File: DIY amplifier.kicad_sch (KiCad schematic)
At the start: 87 parts, among them J1 AudioPlug3, J2 Output, J3 Input, Q1 IRF540N, Q2 IRF540N, Q3 IRF540N, Q4 IRF540N, Q5 DMN2310U, Q6 BC858, Q7 BC858, Q8 BC848, Q9 BC858, SW1 Reset, U1 74LVC1G14, U10 INA181, U11 74LVC2G17, U2 OPA310SxDBV, U3 HIP4081A, U4 74LVC1G17, U5 L7805, U6 L7812, U7 TLV3501AIDBV, U8 MCP6561U

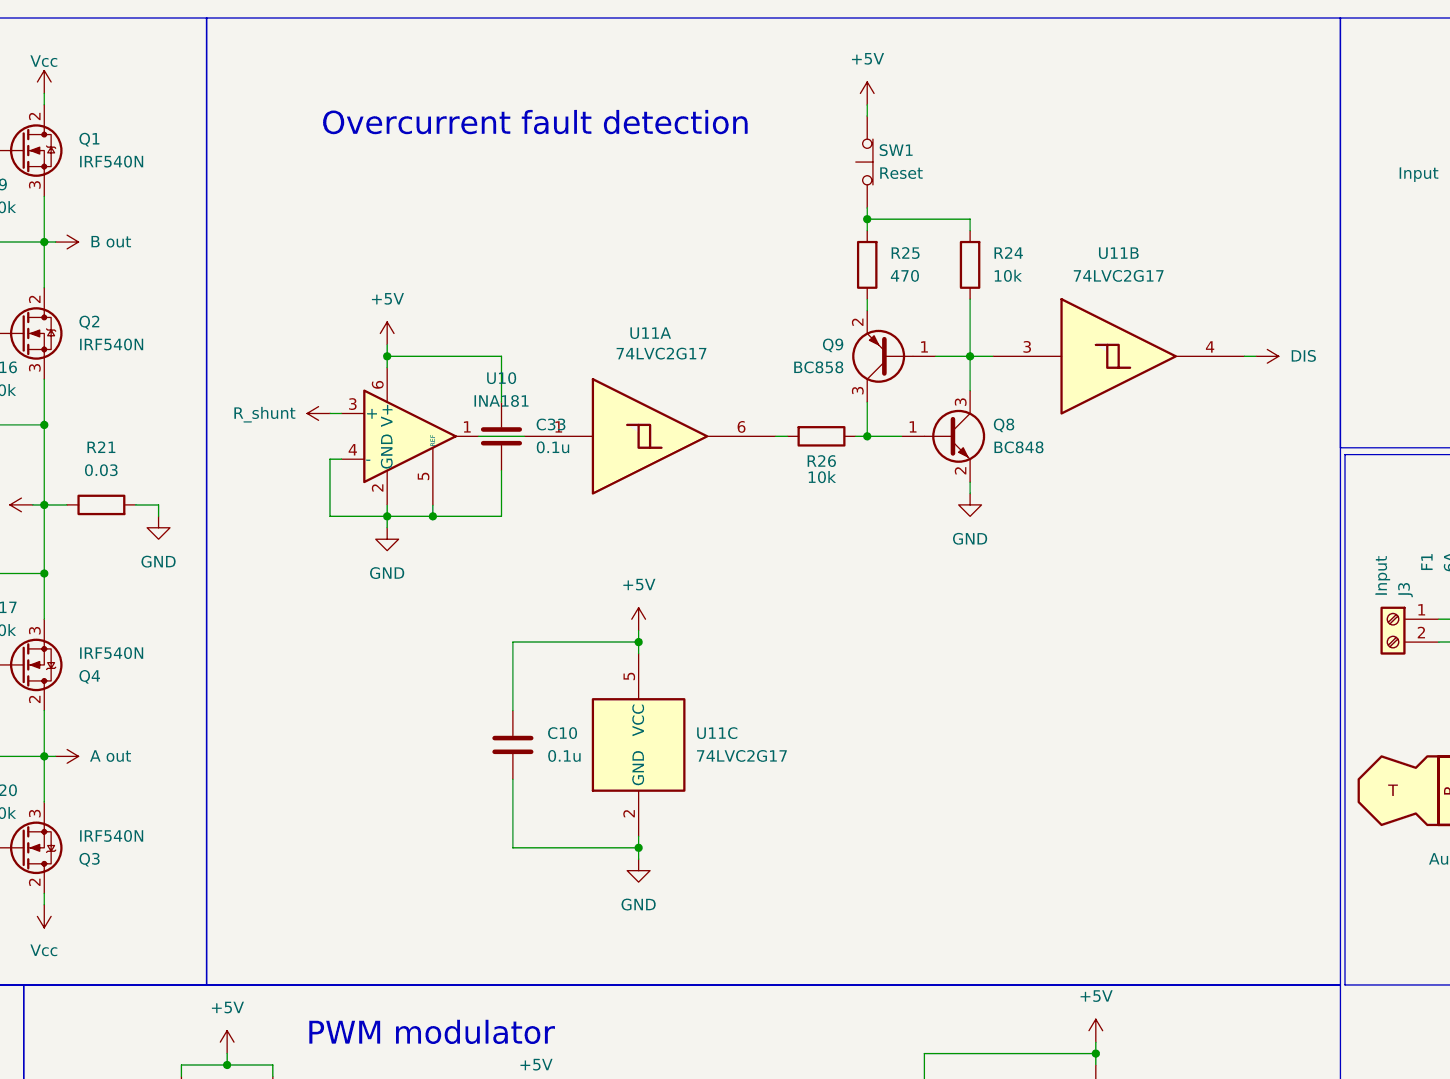
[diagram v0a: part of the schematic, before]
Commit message: Add files via upload
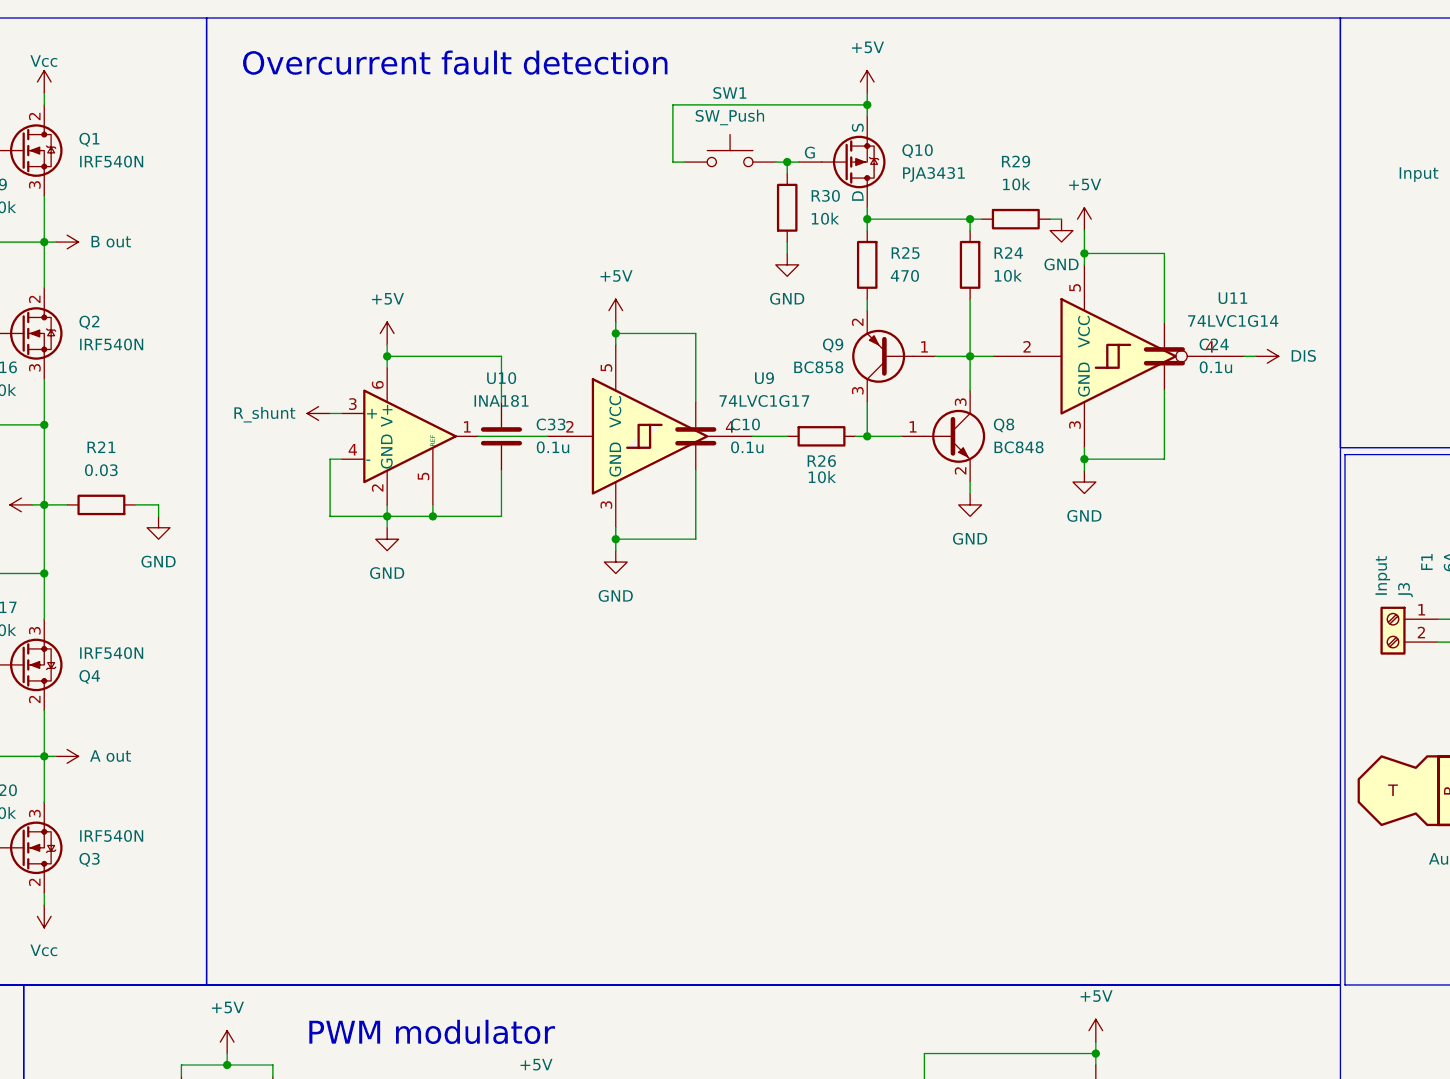
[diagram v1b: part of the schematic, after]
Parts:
- removed SW1: Reset, Button_Switch_THT:SW_PUSH_6mm, symbol Switch:SW_Push_Open
- removed U11: 74LVC2G17, Package_TO_SOT_SMD:SOT-363_SC-70-6, symbol 74xGxx:74LVC2G17
- added C24: 0.1u, Capacitor_SMD:C_0402_1005Metric, symbol Device:C
- added Q10: PJA3431, Package_TO_SOT_SMD:SOT-23-3, symbol Simulation_SPICE:PMOS
- added R29, R30: 10k, Resistor_SMD:R_0603_1608Metric, symbol Device:R
- added SW1: SW_Push, Button_Switch_THT:SW_PUSH_6mm, symbol Switch:SW_Push
- added U11: 74LVC1G14, Package_TO_SOT_SMD:SOT-23-5, symbol 74xGxx:74LVC1G14
- added U9: 74LVC1G17, Package_TO_SOT_SMD:SOT-23-5, symbol 74xGxx:74LVC1G17
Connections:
- net +5V: now also C24.1, Q10.3 (S), SW1.1, U11.5 (VCC), U9.5 (VCC)
- net DIS: now also U11.4
- net GND: now also C24.2, R29.1, R30.2, U11.3 (GND), U9.3 (GND)
- net at U10.1: now also U9.2
- net at Q8.3 (C), Q9.1 (B), R24.1: now also U11.2
- net at R26.2: now also U9.4
- net at R24.2, R25.2: now also Q10.1 (D), R29.2
- new net: Q10.2 (G), R30.1, SW1.2
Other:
- moved on the sheet: C10
